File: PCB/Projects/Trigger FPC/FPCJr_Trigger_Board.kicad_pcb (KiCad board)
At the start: 2 copper layers, 127.6 x 29.7 mm, 10 parts, among them J1 Conn_01x05_Pin, J2 Conn_01x05_Pin, U1 HAL4395, U2 HAL4395, U3 HAL4395, U4 HAL4395

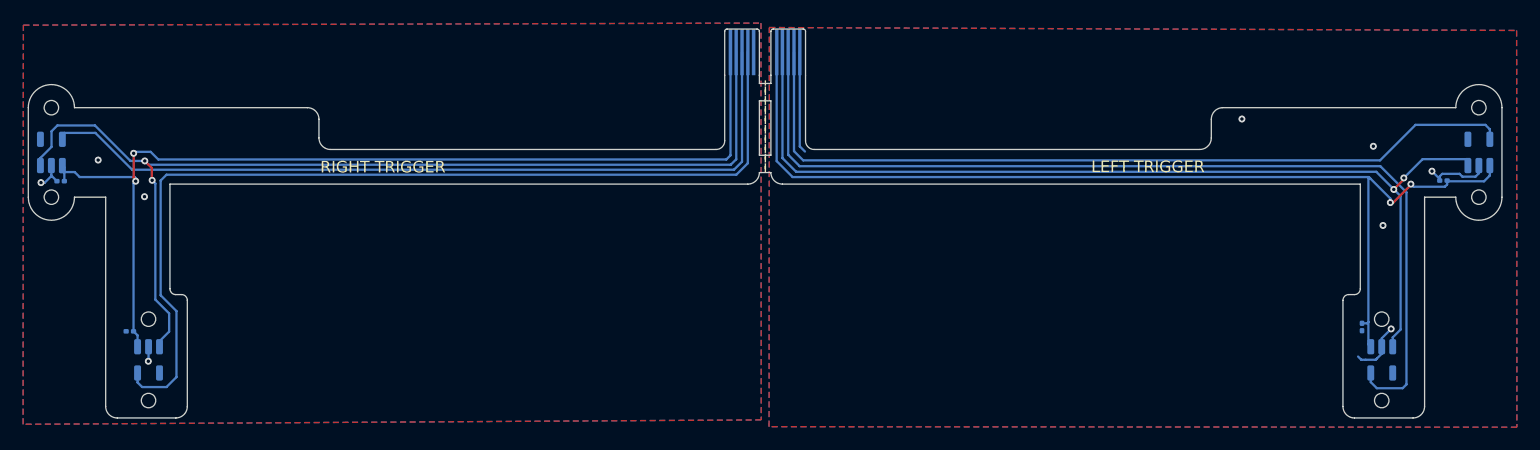
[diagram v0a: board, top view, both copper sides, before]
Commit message: Flex PCB
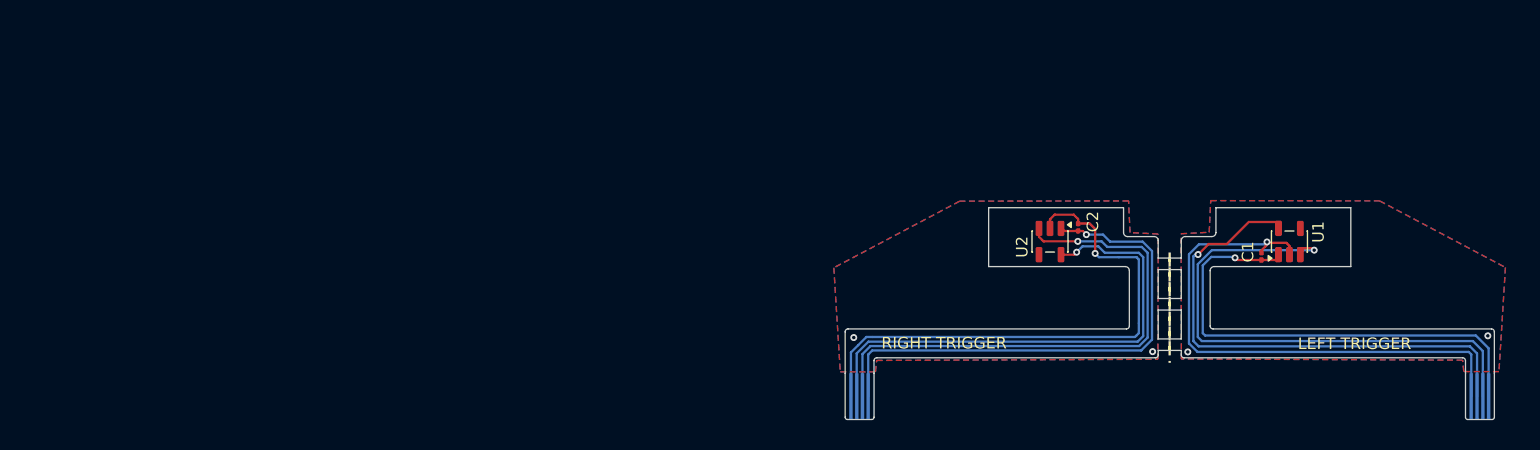
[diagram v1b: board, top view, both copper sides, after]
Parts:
- removed C3, C4: 100n, Capacitor_SMD:C_0201_0603Metric
- removed U3, U4: HAL4395, Package_TO_SOT_SMD:SOT-23-5
- C1, C2, U1, U2: moved to F.Cu
- J1, J2: value Conn_01x05_Pin -> Conn_01x04_Pin; footprint hhl:505110-0592 Ribbon -> hhl:505110-0492 Ribbon
- moved J2 70.5 mm to (280.6, 162.4), turned to -90 degrees
- moved U2 37.9 mm to (243.4, 149.0), turned to -90 degrees
- moved C2 31.9 mm to (245.8, 147.7), turned to -90 degrees
- moved J1 30.4 mm to (226.9, 162.4), turned to -90 degrees
- moved U1 13.0 mm to (264.1, 149.0), turned to 90 degrees
- moved C1 10.6 mm to (261.7, 150.2), turned to -90 degrees
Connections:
- C2 pad 1: GNDL -> GND
- C2 pad 2: +3V3L -> +3V3
- J1 pad 1: +3V3L -> +3V3
- J1 pad 2: TRIGGER_EN_L -> TRIGGER_EN_R
- J1 pad 3: ADC_3 -> ADC_1
- J1 pad 4: ADC_2 -> GND
- J2 pad 1: +3V3 -> +3V3L
- J2 pad 2: TRIGGER_EN_R -> TRIGGER_EN_L
- J2 pad 4: ADC_1 -> GNDL
- U1 pad 5: ADC_3 -> ADC_0
- U2 pad 1: +3V3L -> +3V3
- U2 pad 2: GNDL -> GND
- U2 pad 3: TRIGGER_EN_L -> TRIGGER_EN_R
- U2 pad 5: ADC_2 -> ADC_1
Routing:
- net ADC_3: track 84.7 -> 0.00 mm
- net ADC_2: track 71.5 -> 0.00 mm
- net +3V3L: track 90.9 -> 42.7 mm, vias 2 -> 1
- net TRIGGER_EN_R: track 91.1 -> 47.0 mm, vias 2 -> 1
- net GND: track 3.99 -> 47.5 mm, vias 4 -> 3
- net +3V3: track 86.6 -> 45.1 mm, vias 2 -> 1
- net ADC_1: track 83.4 -> 43.9 mm, vias 0 -> 1
- net TRIGGER_EN_L: track 85.5 -> 47.4 mm, vias 2 -> 1
- net GNDL: track 19.5 -> 47.5 mm, vias 5 -> 3
- net ADC_0: track 70.4 -> 45.1 mm, vias 0 -> 1
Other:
- board size 127.6 x 29.7 mm -> 56.2 x 14.3 mm
